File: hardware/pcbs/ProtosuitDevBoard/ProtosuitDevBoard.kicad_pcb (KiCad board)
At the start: 4 copper layers, 145 x 110 mm, 36 parts, among them J1 PWR IN, J10 Left Ear, J11 Right Ear, J12 Microphone input, J13 Display I2C, J14 Extra I2C, J15 Boop Sensor I2C, J16 FAN, J17 DHT22 sensor, J2 RPi Out, J3 Front Left, J4 Back Right, J5 Back Left, J6 Front Right, J7 Upper Arch, J8 Left Fin, J9 Right Fin, Q1 2N3904, U1 DC-DC 5v 5A TPS54X60, U2 DC-DC 5v 8A CRDC2580, U3 Teensy 4.0, U4 Wemos D1 Mini ESP32, U7 MPU6050 Gyroscope

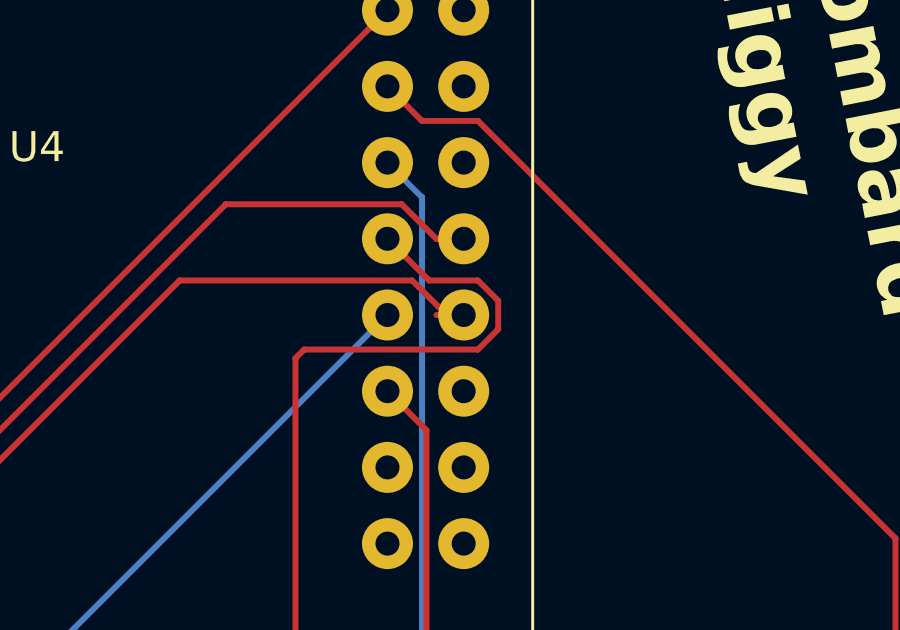
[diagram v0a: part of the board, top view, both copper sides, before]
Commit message: Updated documentation
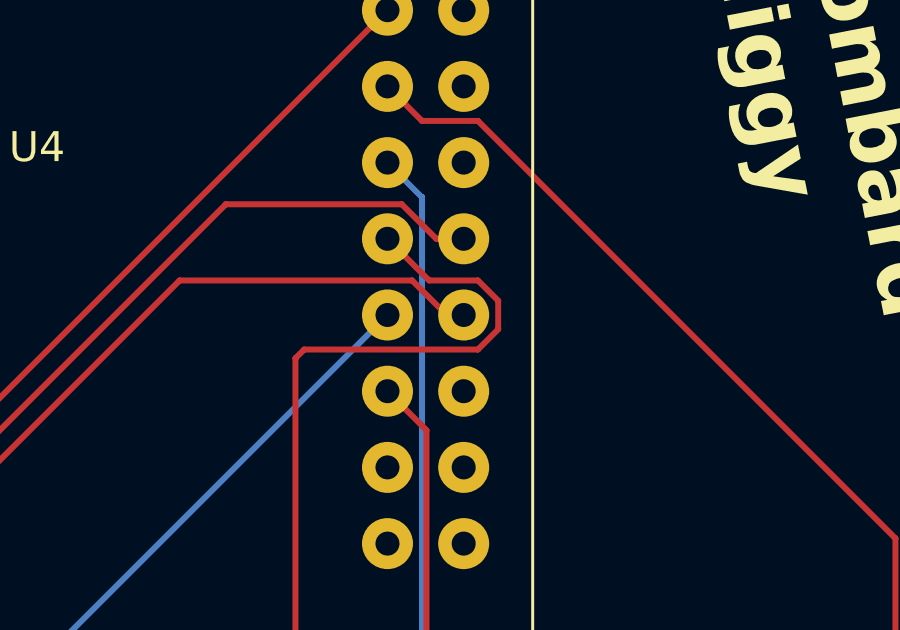
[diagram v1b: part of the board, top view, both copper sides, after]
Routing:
- net Net-(J16-Pin_3): track 93.5 -> 92.6 mm
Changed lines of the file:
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@@
-	)
-	(segment
-		(start 195.24 68.38)
-		(end 194.32776 68.38)
-		(width 0.2)
-		(layer "F.Cu")
-		(net 66)
 	)
 	(segment
